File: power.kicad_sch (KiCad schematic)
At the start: 14 parts, among them J3 USB4105-GF-A, U1 NCP1117-3.3_SOT223

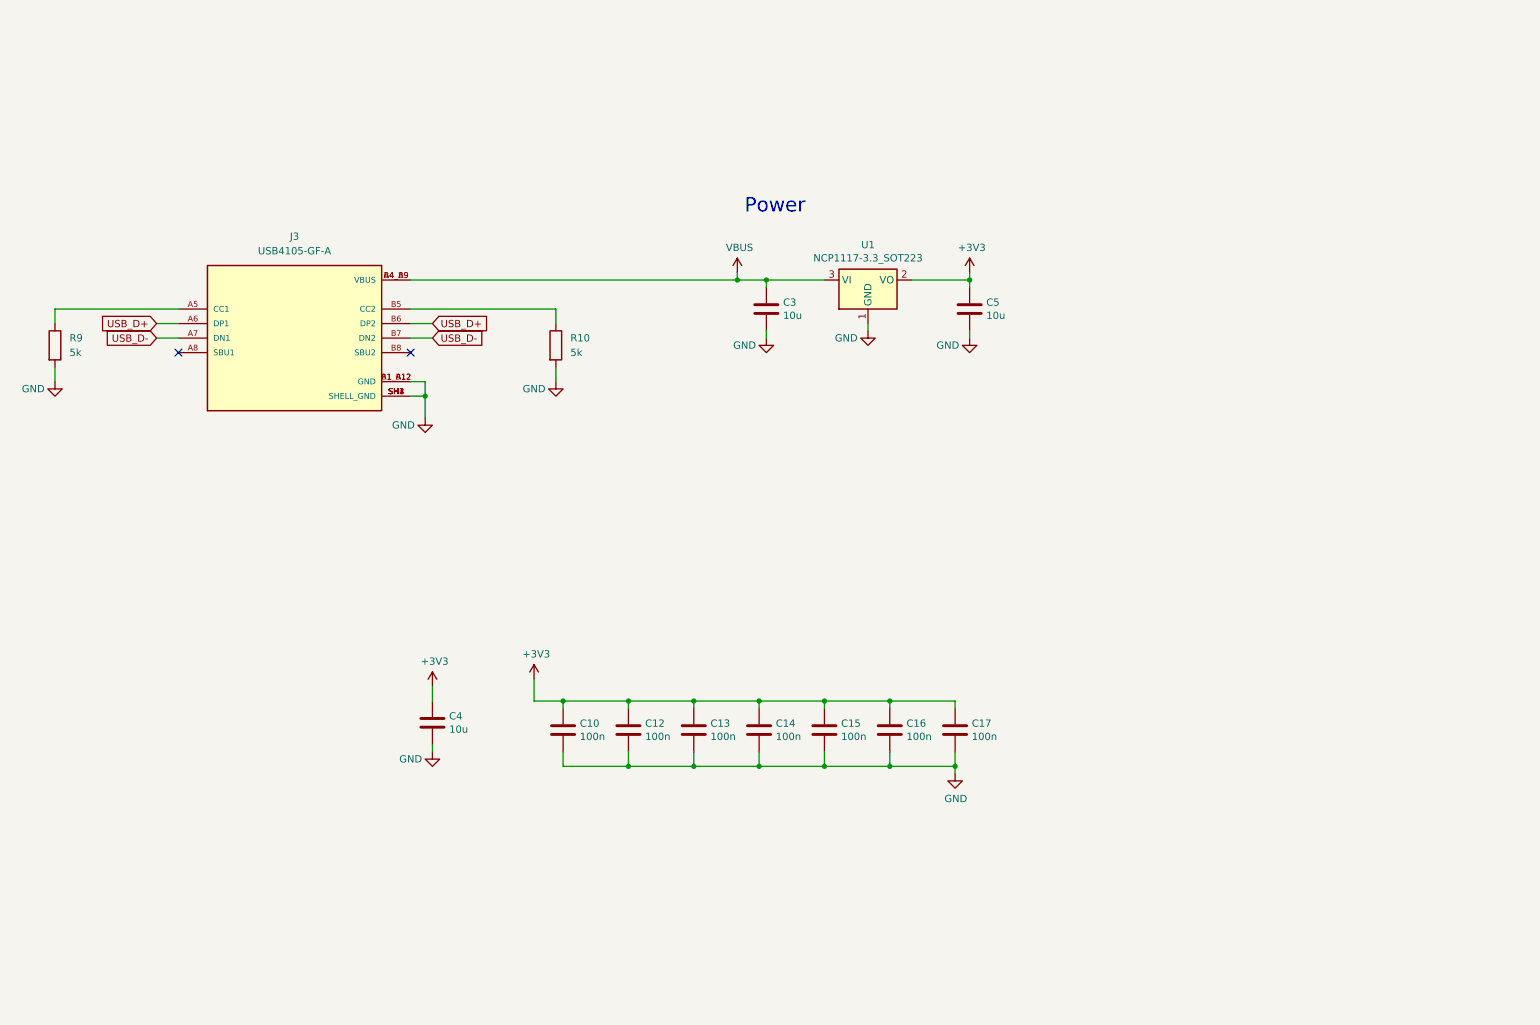
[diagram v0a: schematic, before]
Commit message: WIP - Started implementation of selector switch
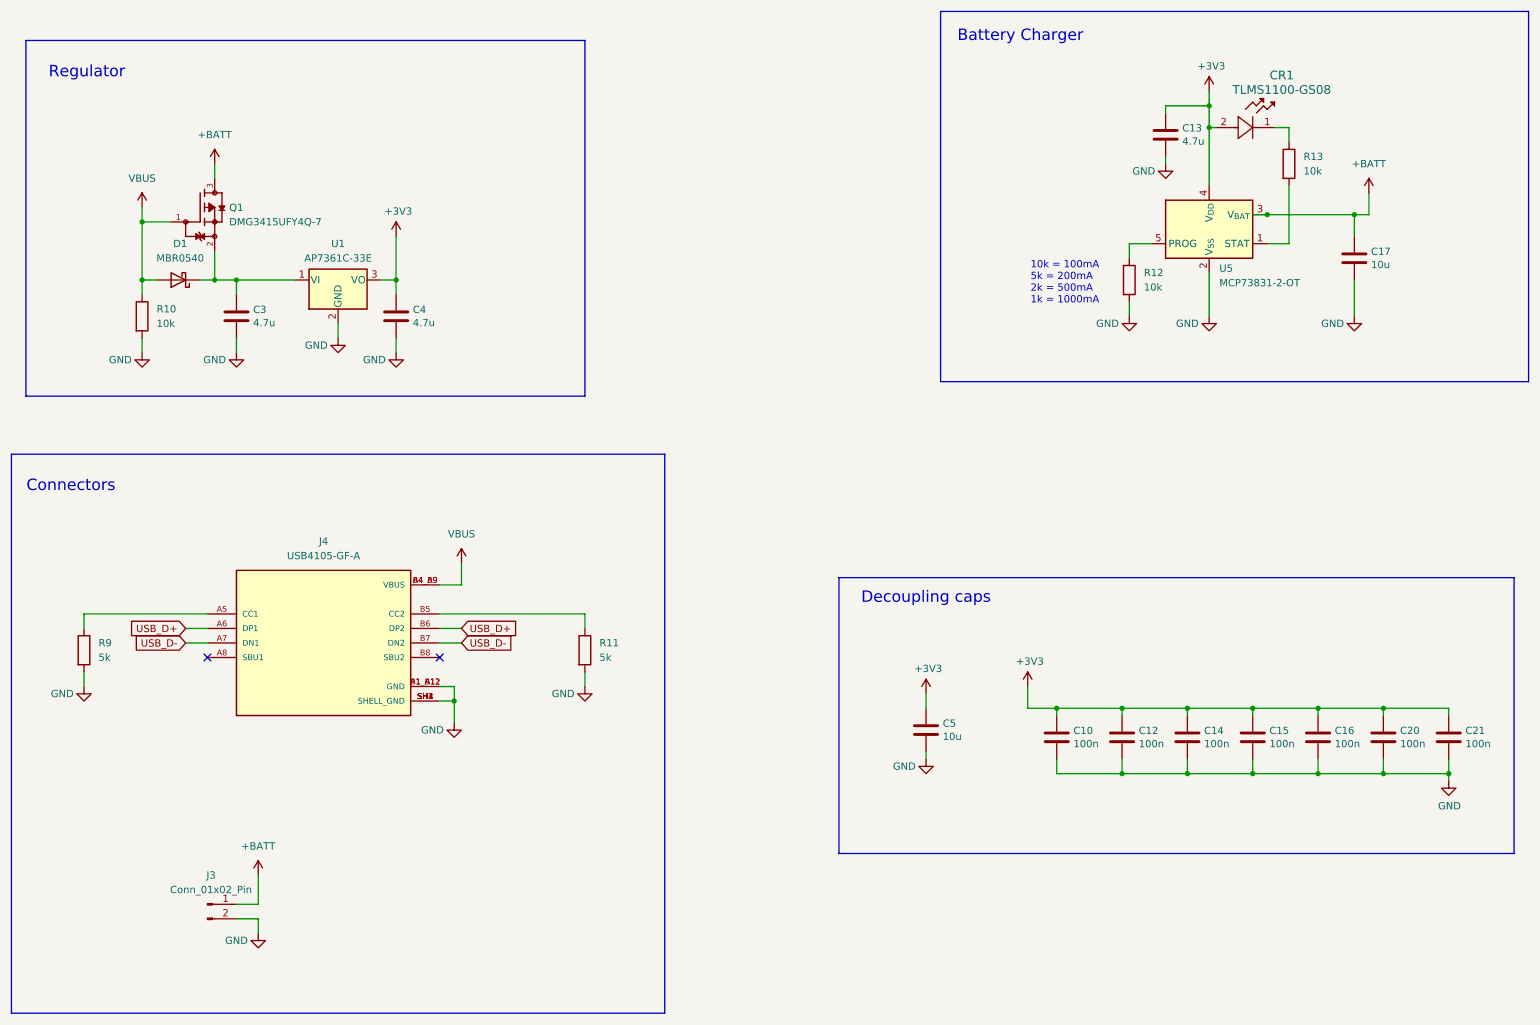
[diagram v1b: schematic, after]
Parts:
- removed J3: USB4105-GF-A, duso:GCT_USB4105-GF-A, symbol USB4105-GF-A:USB4105-GF-A
- removed U1: NCP1117-3.3_SOT223, Package_TO_SOT_SMD:SOT-223-3_TabPin2, symbol Regulator_Linear:NCP1117-3.3_SOT223
- added C20, C21: 100n, Capacitor_SMD:C_0402_1005Metric, symbol Device:C
- added CR1: TLMS1100-GS08, LED_VISHAY_TLMX1100_VIS, symbol TLMS1100-GS08:TLMS1100-GS08
- added D1: MBR0540, Diode_SMD:D_SOD-123, symbol Diode:MBR0540
- added J3: Conn_01x02_Pin, Connector_JST:JST_PH_B2B-PH-K_1x02_P2.00mm_Vertical, symbol Connector:Conn_01x02_Pin
- added J4: USB4105-GF-A, duso:GCT_USB4105-GF-A, symbol USB4105-GF-A:USB4105-GF-A
- added Q1: DMG3415UFY4Q-7, duso:TRANS_DMG3415UFY4Q-7, symbol DMG3415UFY4Q-7:DMG3415UFY4Q-7
- added R11: 5k, Resistor_SMD:R_0603_1608Metric, symbol Device:R
- added R12, R13: 10k, Resistor_SMD:R_0603_1608Metric, symbol Device:R
- added U1: AP7361C-33E, Package_TO_SOT_SMD:SOT-223-3_TabPin2, symbol Regulator_Linear:AP7361C-33E
- added U5: MCP73831-2-OT, Package_TO_SOT_SMD:SOT-23-5, symbol Battery_Management:MCP73831-2-OT
- C13: value 100n -> 4.7u
- C17: value 100n -> 10u
- C3, C4: value 10u -> 4.7u; footprint Capacitor_SMD:C_0805_2012Metric -> Capacitor_SMD:C_0402_1005Metric
- R10: value 5k -> 10k
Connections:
- net +3V3: now also C20.1, C21.1, CR1.2, U1.3 (VO), U5.4 (V_{DD}); no longer C17.1
- net GND: now also C20.2, C21.2, J3.2 (Pin_2), J4.A1_B12 (GND), J4.B1_A12 (GND), J4.SH1 (SHELL_GND), J4.SH2 (SHELL_GND), J4.SH3 (SHELL_GND), J4.SH4 (SHELL_GND), R11.2, R12.2, U1.2 (GND), U5.2 (V_{SS})
- net USB_D+: now also J4.A6 (DP1), J4.B6 (DP2)
- net USB_D-: now also J4.A7 (DN1), J4.B7 (DN2)
- net VBUS: now also R10.1, D1.2 (A), J4.A4_B9 (VBUS), J4.B4_A9 (VBUS), Q1.1; no longer C3.1
- net at R9.1: now also J4.A5 (CC1)
- new net: CR1.1, R13.1
- new net: C3.1, D1.1 (K), Q1.2, U1.1 (VI)
- new net: J4.B5 (CC2), R11.1
- new net: R12.1, U5.5 (PROG)
- new net: R13.2, U5.1 (STAT)
- new net +BATT: C17.1, J3.1 (Pin_1), Q1.3, U5.3 (V_{BAT})
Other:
- note added: "10k = 100mA 5k = 200mA 2k = 500mA 1k = 1000mA"
- note added: "Battery Charger"
- note added: "Connectors"
- note added: "Decoupling caps"
- note added: "Regulator"
- note removed: "Power"
